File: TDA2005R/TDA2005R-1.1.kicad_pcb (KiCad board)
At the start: 2 copper layers, 71.8 x 83.8 mm, 29 parts, among them J1 6-pole_dual_potentiometer_hea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, U1 4-pole_RL-input_screw_terminal, U2 TDA2005, U3 4-pole_RL-output_screw_termin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, U4 2-pole_power_in_screw_terminal

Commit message: kicad6
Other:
- net class 30 removed
- net class 50 removed
- net class Default removed

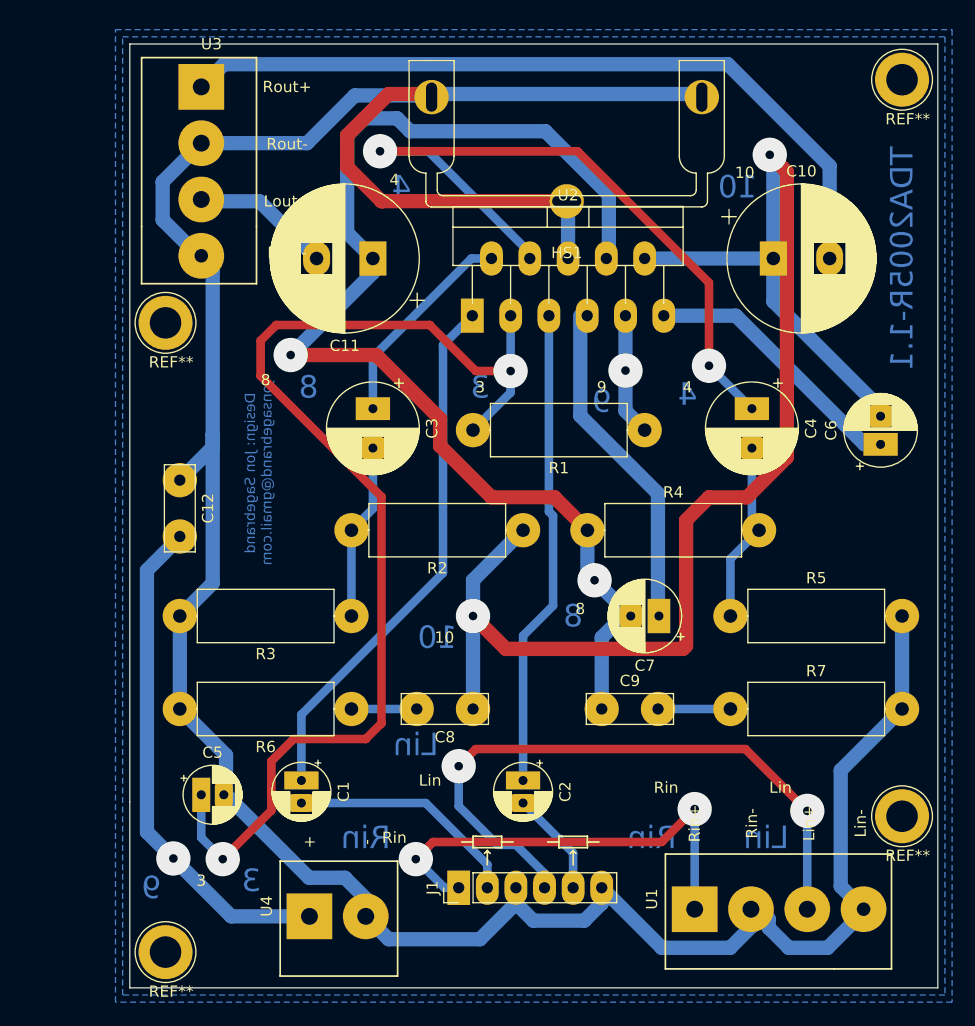
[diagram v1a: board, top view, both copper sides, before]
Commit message: amplifier
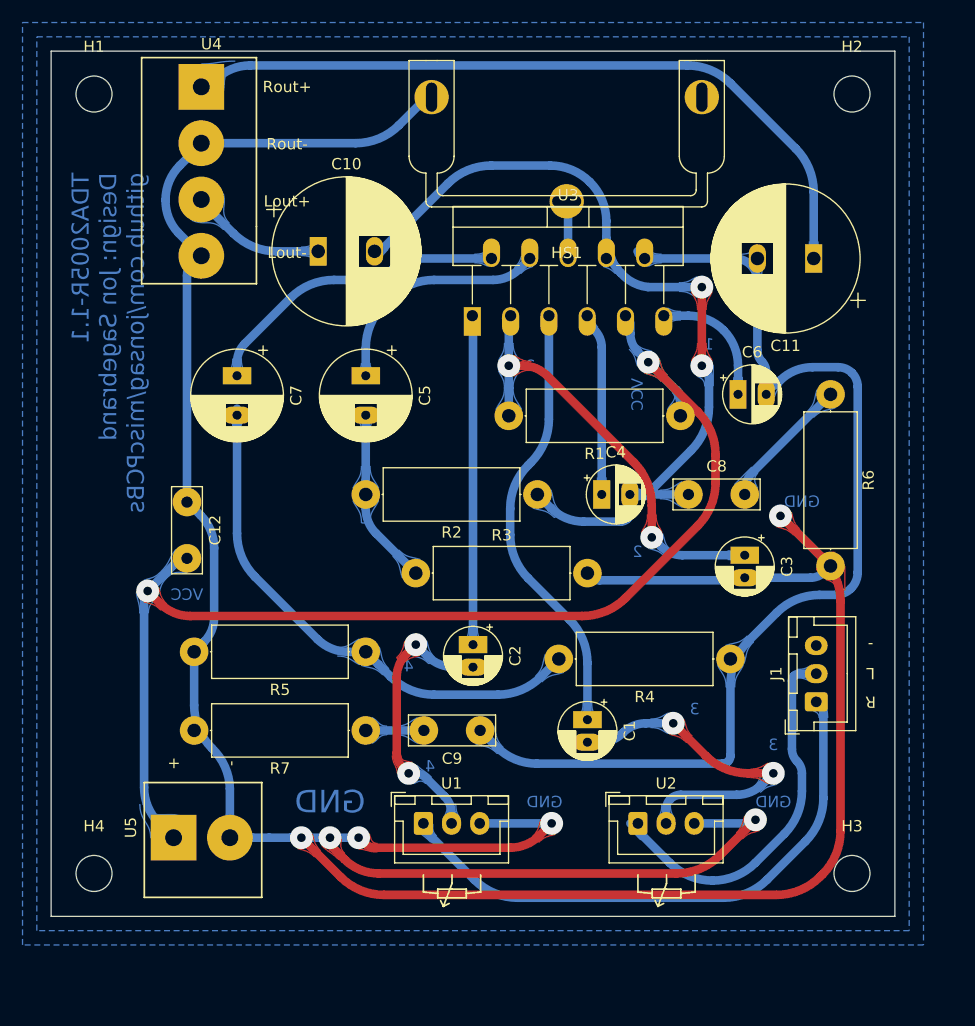
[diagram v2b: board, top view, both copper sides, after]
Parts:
- removed REF** (x4): TestPoint_Loop_D3.80mm_Drill2.8mm, TestPoint:TestPoint_Loop_D3.80mm_Drill2.8mm
- added H1: MountingHole, MountingHole:MountingHole_3.2mm_M3, F.Cu at (152.6, -112.9)
- added H2: MountingHole, MountingHole:MountingHole_3.2mm_M3, F.Cu at (220.0, -112.9)
- added H3: MountingHole, MountingHole:MountingHole_3.2mm_M3, F.Cu at (220.0, -43.7)
- added H4: MountingHole, MountingHole:MountingHole_3.2mm_M3, F.Cu at (152.6, -43.7)
- added U2: Vol L, My_Headers:3-pin JST Potentiometer, F.Cu at (200.9, -48.2)
- C3: value 220u -> 10u; footprint My_Misc:CP_Radial_D8.0mm_P3.50mm_large -> My_Misc:CP_Radial_D5.0mm_P2.00mm_larger
- C4: value 220u -> 100u; footprint My_Misc:CP_Radial_D8.0mm_P3.50mm_large -> My_Misc:CP_Radial_D5.0mm_P2.50mm_larger_pads
- C5: value 10u -> 220u; footprint My_Misc:CP_Radial_D5.0mm_P2.00mm_larger -> My_Misc:CP_Radial_D8.0mm_P3.50mm_large
- C6: footprint My_Misc:CP_Radial_D6.3mm_P2.50mm_large -> My_Misc:CP_Radial_D5.0mm_P2.50mm_larger_pads
- C7: value 100u -> 220u; footprint My_Misc:CP_Radial_D6.3mm_P2.50mm_large -> My_Misc:CP_Radial_D8.0mm_P3.50mm_large
- J1: value 6-pole_dual_potentiometer_header -> Audio In; footprint My_Headers:6-pin_dual_potentiometer_header_large -> My_Headers:3-pin JST Audio
- R3: renamed from R5; value 33R -> 3R3
- R5: renamed from R3; value 33R -> 3R3
- U1: value 4-pole_RL-input_screw_terminal -> Vol R; footprint My_Parts:4-pole_screw_terminal_RL_input -> My_Headers:3-pin JST Potentiometer
- U4: renamed from U3; value 4-pole_RL-output_screw_terminal -> Speakers
- U5: renamed from U4; value 2-pole_power_in_screw_terminal -> Power In
- moved C7 43.1 mm to (165.3, -87.9), turned to -90 degrees
- moved C10 40.4 mm to (172.6, -99.0)
- moved C5 40.0 mm to (176.8, -87.9), turned to -90 degrees
- moved C11 39.1 mm to (216.6, -98.3)
- moved J1 35.8 mm to (216.8, -59.0)
- moved C3 35.5 mm to (210.4, -72.0)
- moved R6 29.3 mm to (218.1, -86.3), turned to -90 degrees
- moved R3 28.2 mm to (181.2, -70.4)
- moved C1 26.0 mm to (196.5, -57.4)
- moved U1 25.3 mm to (181.9, -48.2), turned to 0 degrees
- moved R4 21.7 mm to (209.2, -62.8)
- moved C8 20.5 mm to (205.4, -77.4)
- moved C4 15.4 mm to (197.7, -77.4), turned to 0 degrees
- moved U5 13.9 mm to (159.7, -46.9)
- moved C6 13.4 mm to (209.8, -86.3), turned to 0 degrees
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- renumbered C9 to C8, C8 to C9, R4 to R2, R2 to R4, R7 to R6, R6 to R7, U2 to U3
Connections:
- C10 pad 1: Net-(C10-Pad1) -> Lout
- C10 pad 2: Rout -> Net-(C10-Pad2)
- C11 pad 1: Net-(C11-Pad1) -> Rout
- C11 pad 2: Lout -> Net-(C11-Pad2)
- C3 pad 2: Net-(C3-Pad2) -> GND
- C4 pad 2: Net-(C4-Pad2) -> Net-(C10-Pad2)
- C5 pad 2: GND -> Net-(C5-Pad2)
- C6 pad 2: Net-(C10-Pad1) -> Net-(C11-Pad2)
- C7 pad 2: Net-(C11-Pad1) -> Net-(C7-Pad2)
- C8 pad 1: Net-(C11-Pad1) -> Net-(C10-Pad2)
- C9 pad 1: Net-(C10-Pad1) -> Net-(C11-Pad2)
- J1 pad 2: Net-(C1-Pad2) -> Lin
- R1 pad 2: Net-(C5-Pad1) -> Net-(C3-Pad1)
- R2 pad 1: Net-(C11-Pad1) -> Net-(C10-Pad2)
- R2 pad 2: Net-(C4-Pad2) -> Net-(C5-Pad2)
- R3 pad 1: Net-(C4-Pad2) -> Net-(C5-Pad2)
- R4 pad 1: Net-(C10-Pad1) -> Net-(C11-Pad2)
- R4 pad 2: Net-(C3-Pad2) -> Net-(C7-Pad2)
- R5 pad 1: Net-(C3-Pad2) -> Net-(C7-Pad2)
- U1 pad 2: GND -> Net-(C2-Pad2)
- U1 pad 3: Lin -> GND
- U3 pad 1: Net-(C1-Pad1) -> Net-(C2-Pad1)
- U3 pad 10: Net-(C10-Pad1) -> Net-(C11-Pad2)
- U3 pad 2: Net-(C3-Pad1) -> Net-(C7-Pad1)
- U3 pad 3: Net-(C5-Pad1) -> Net-(C3-Pad1)
- U3 pad 4: Net-(C4-Pad1) -> Net-(C5-Pad1)
- U3 pad 5: Net-(C2-Pad1) -> Net-(C1-Pad1)
- U3 pad 7: Net-(C7-Pad1) -> Net-(C4-Pad1)
- U3 pad 8: Net-(C11-Pad1) -> Net-(C10-Pad2)
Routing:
- net Net-(C10-Pad1): track 126.6 -> 0.00 mm, vias 2 -> 0
- net Net-(C11-Pad1): track 108.7 -> 0.00 mm, vias 2 -> 0
- net Net-(C11-Pad2): track 0.00 -> 93.7 mm
- net Net-(C5-Pad1): track 102.6 -> 21.3 mm, vias 2 -> 0
- net Net-(C10-Pad2): track 0.00 -> 75.9 mm, vias 0 -> 2
- net +15V: track 55.8 -> 106.6 mm
- net Net-(C4-Pad1): track 64.3 -> 15.7 mm, vias 2 -> 0
- net Net-(C7-Pad2): track 0.00 -> 47.1 mm
- net GND: track 260.1 -> 288.2 mm, vias 0 -> 6
- net Lin: track 58.1 -> 33.7 mm, vias 2 -> 0
- net Net-(C3-Pad1): track 18.1 -> 39.3 mm, vias 0 -> 2
- net Net-(C4-Pad2): track 16.2 -> 0.00 mm
- net Net-(C5-Pad2): track 0.00 -> 15.7 mm
- net Net-(C3-Pad2): track 15.7 -> 0.00 mm
- net Net-(C2-Pad2): track 9.37 -> 24.6 mm, vias 0 -> 2
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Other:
- board size 71.8 x 83.8 mm -> 74.9 x 76.8 mm
- board text added: "1"
- board text added: "2"
- board text added: "GND"
- board text added: "TDA2005R-1.1 Design: Jon Sagebrand github.com/jonsag/miscPCBs"
- board text added: "VCC"
- board text removed: "10"
- board text removed: "8"
- board text removed: "9"
- board text removed: "Design: Jon Sagebrand jonsagebrand@gmail.com"
- board text removed: "Lin"
- board text removed: "Rin"
- board text removed: "TDA2005R-1.1"
